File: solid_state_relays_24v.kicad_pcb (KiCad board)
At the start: 2 copper layers, 120 x 90 mm, 69 parts, among them J1 1190297, J2 1190297, J3 1190297, J4 1190297, J5 1190297, J6 1190297, J7 1190297, J8 1190297, Q1 IRF4905PBF, Q2 IRF4905PBF, Q3 IRF4905PBF, Q4 IRF4905PBF, Q5 IRF4905PBF, Q6 IRF4905PBF, Q7 IRF4905PBF, Q8 IRF4905PBF

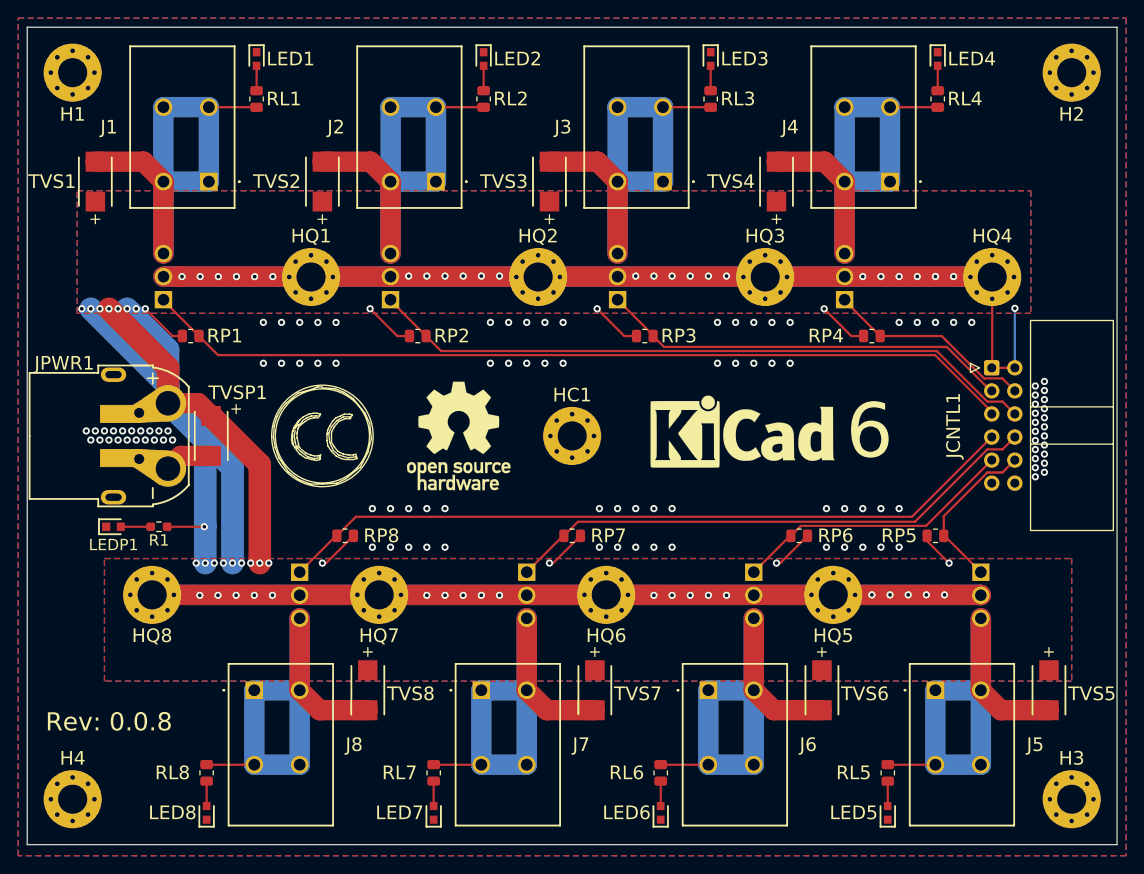
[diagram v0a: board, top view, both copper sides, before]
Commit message: v0.0.10-pre2
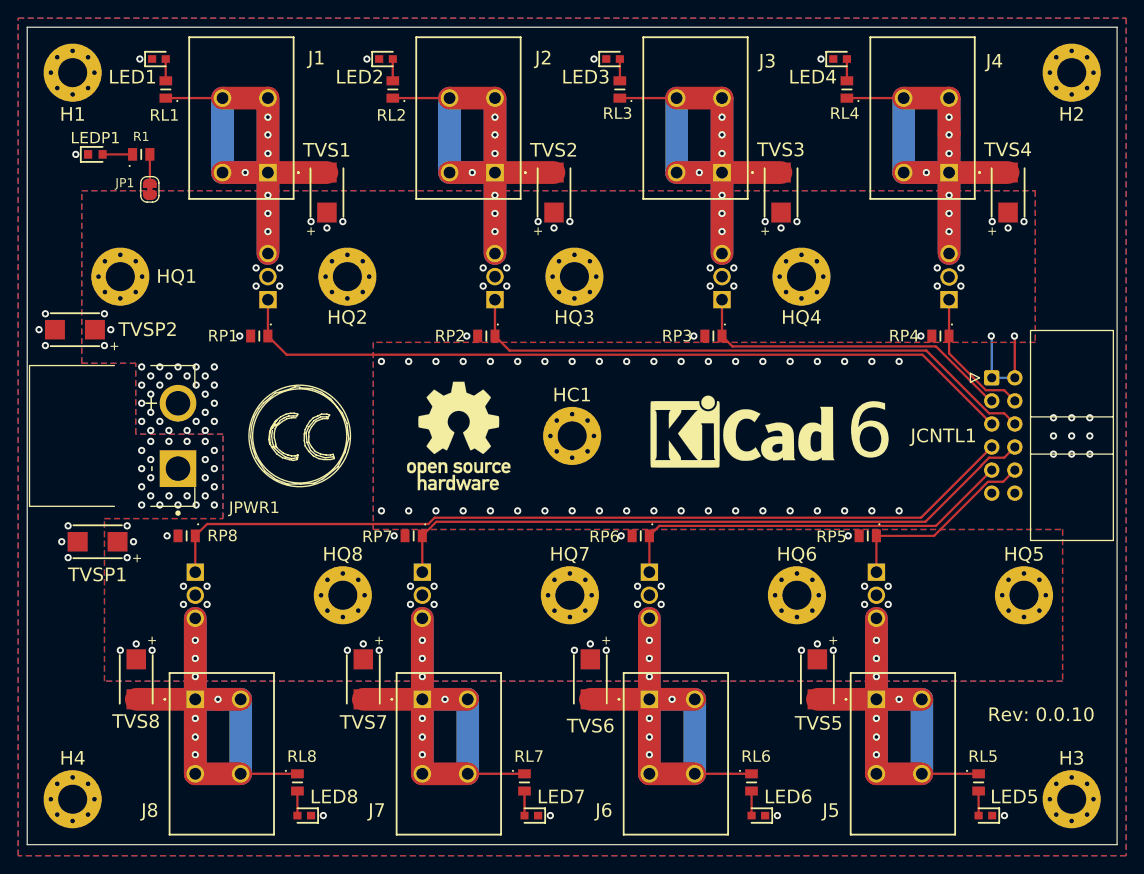
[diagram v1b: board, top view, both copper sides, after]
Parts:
- added JP1: SolderJumper_2_Bridged, Jumper:SolderJumper-2_P1.3mm_Bridged_RoundedPad1.0x1.5mm, F.Cu at (63.5, 67.8)
- added TVSP2: SM6T30AY, dragon_mobile:SMBJ36CATR, F.Cu at (55.2, 83.3)
- JPWR1: value XT60PW-M_Kombifootprint -> XT60PW-M; footprint dragon_mobile:Amass_XT60PW-M_Kombifootprint -> dragon_mobile:XT60PWM
- R1: value 1k2 -> 1k5; footprint Resistor_SMD:R_0603_1608Metric_Pad0.98x0.95mm_HandSolder -> dragon_mobile:RESC2012X65N
- RL1, RL2, RL3, RL4, RL5, RL6, RL7, RL8: value 1k2 -> 1k5; footprint Resistor_SMD:R_0805_2012Metric -> dragon_mobile:RESC2012X65N
- RP1, RP2, RP3, RP4, RP5, RP6, RP7, RP8: footprint Resistor_SMD:R_0805_2012Metric -> dragon_mobile:RESC2012X65N
- moved LEDP1 41.0 mm to (57.5, 64.0)
- moved R1 41.0 mm to (62.5, 64.0)
- moved TVS1 25.5 mm to (83.0, 68.2)
- moved TVS2 25.5 mm to (108.0, 68.2)
- moved TVS3 25.5 mm to (133.0, 68.2)
- moved TVS4 25.5 mm to (158.0, 68.2)
- moved TVS5 25.5 mm to (137.0, 121.8)
- moved TVS6 25.5 mm to (112.0, 121.8)
- moved TVS7 25.5 mm to (87.0, 121.8)
- moved TVS8 25.5 mm to (62.0, 121.8)
- moved HQ1 21.0 mm to (60.2, 77.5)
- moved HQ2 21.0 mm to (85.2, 77.5)
- moved HQ3 21.0 mm to (110.2, 77.5)
- moved HQ4 21.0 mm to (135.2, 77.5)
- moved HQ5 21.0 mm to (159.8, 112.5)
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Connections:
- R1 pad 2: +BATT -> Net-(JP1-Pad2)
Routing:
- net +BATT: track 531.0 -> 11.7 mm, vias 70 -> 99
- net OUT3: track 55.9 -> 70.2 mm, vias 0 -> 7
- net OUT2: track 55.9 -> 70.2 mm, vias 0 -> 7
- net OUT1: track 55.9 -> 70.2 mm, vias 0 -> 7
- net OUT8: track 55.9 -> 70.2 mm, vias 0 -> 7
- net OUT7: track 55.9 -> 70.2 mm, vias 0 -> 7
- net OUT6: track 55.9 -> 70.2 mm, vias 0 -> 7
- net OUT4: track 55.9 -> 70.2 mm, vias 0 -> 7
- net OUT5: track 55.9 -> 70.2 mm, vias 0 -> 7
- net /a7: track 59.8 -> 73.3 mm
- net /a6: track 31.2 -> 44.7 mm
- net /a8: track 82.3 -> 95.8 mm
- net /a3: track 45.2 -> 36.5 mm
- net /a2: track 73.9 -> 65.2 mm
- net /a1: track 96.3 -> 87.7 mm
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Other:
- board text added: "Rev: 0.0.10"
- board text added: "https://github.com/dragon-mobile/solid_state_relays_24v"
- board text added: "© 2022 Michael Cummings"
- board text removed: "Rev: 0.0.8"
